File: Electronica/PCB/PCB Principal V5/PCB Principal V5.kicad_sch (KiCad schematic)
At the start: 17 parts, among them J1 Conexion Sensores, J12 TP, J2 Power Monster, J3 On/Off General, J4 Power Input 2, J5 IDC Placa Botones, J6 Power Input 1, SW1 On/Off Motores

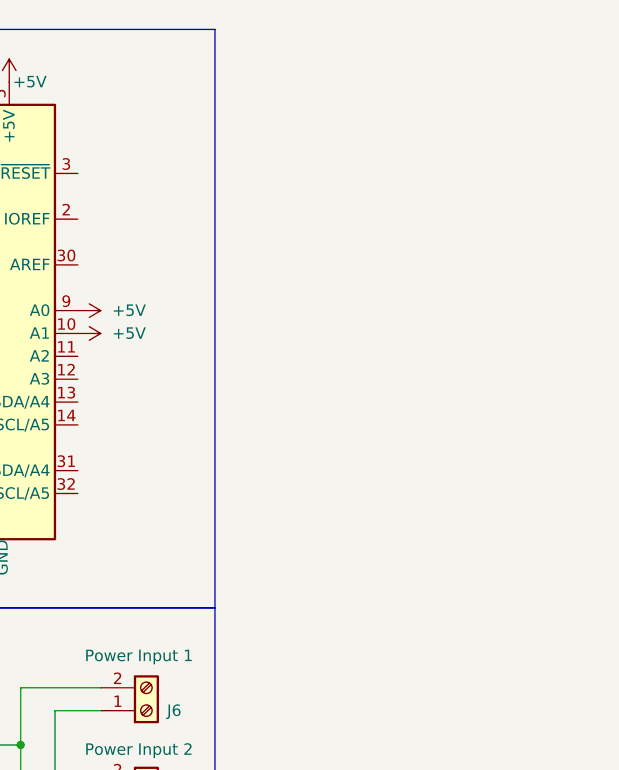
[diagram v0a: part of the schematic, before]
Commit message: ok
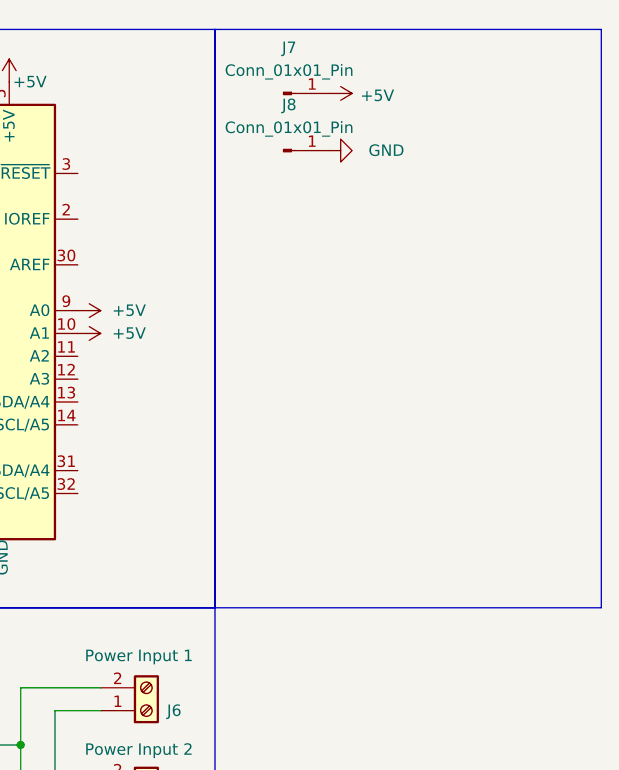
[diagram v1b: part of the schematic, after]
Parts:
- added J7, J8: Conn_01x01_Pin, Connector_PinHeader_2.54mm:PinHeader_1x01_P2.54mm_Vertical, symbol Connector:Conn_01x01_Pin
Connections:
- net +5V: now also J7.1 (Pin_1)
- net GND: now also J8.1 (Pin_1)

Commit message: .
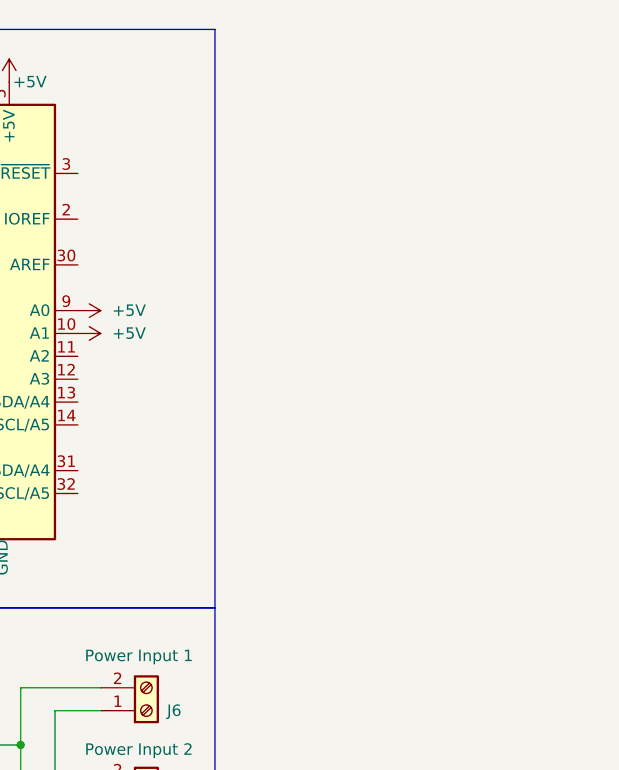
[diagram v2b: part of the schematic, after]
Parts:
- removed J7, J8: Conn_01x01_Pin, Connector_PinHeader_2.54mm:PinHeader_1x01_P2.54mm_Vertical, symbol Connector:Conn_01x01_Pin

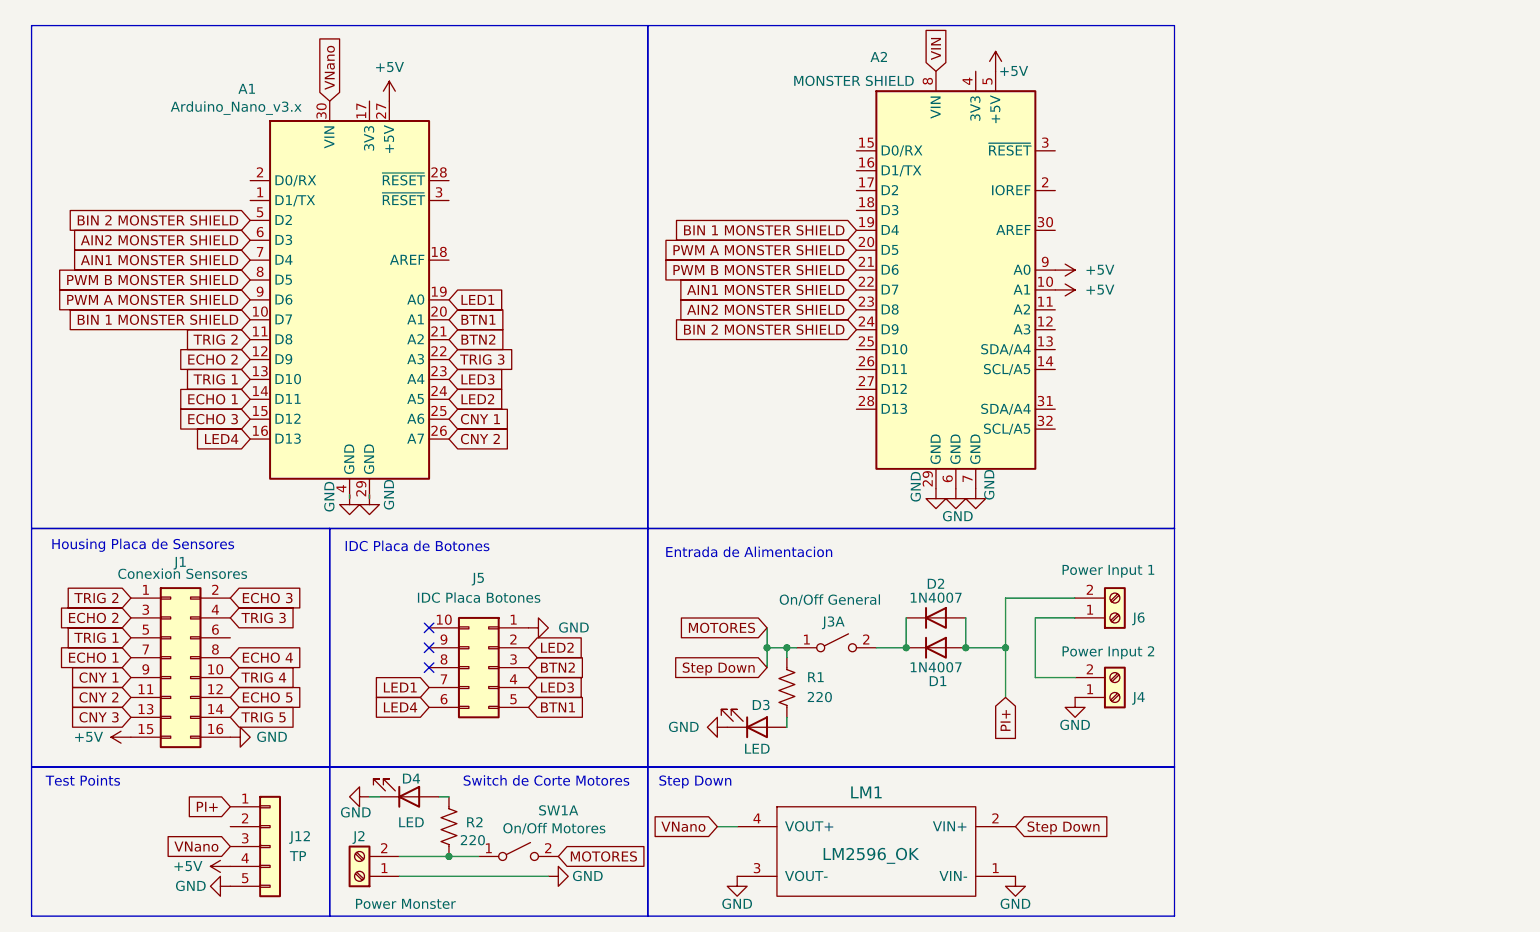
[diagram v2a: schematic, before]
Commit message: PCB V5 LINDA HERMOSA DIVINA
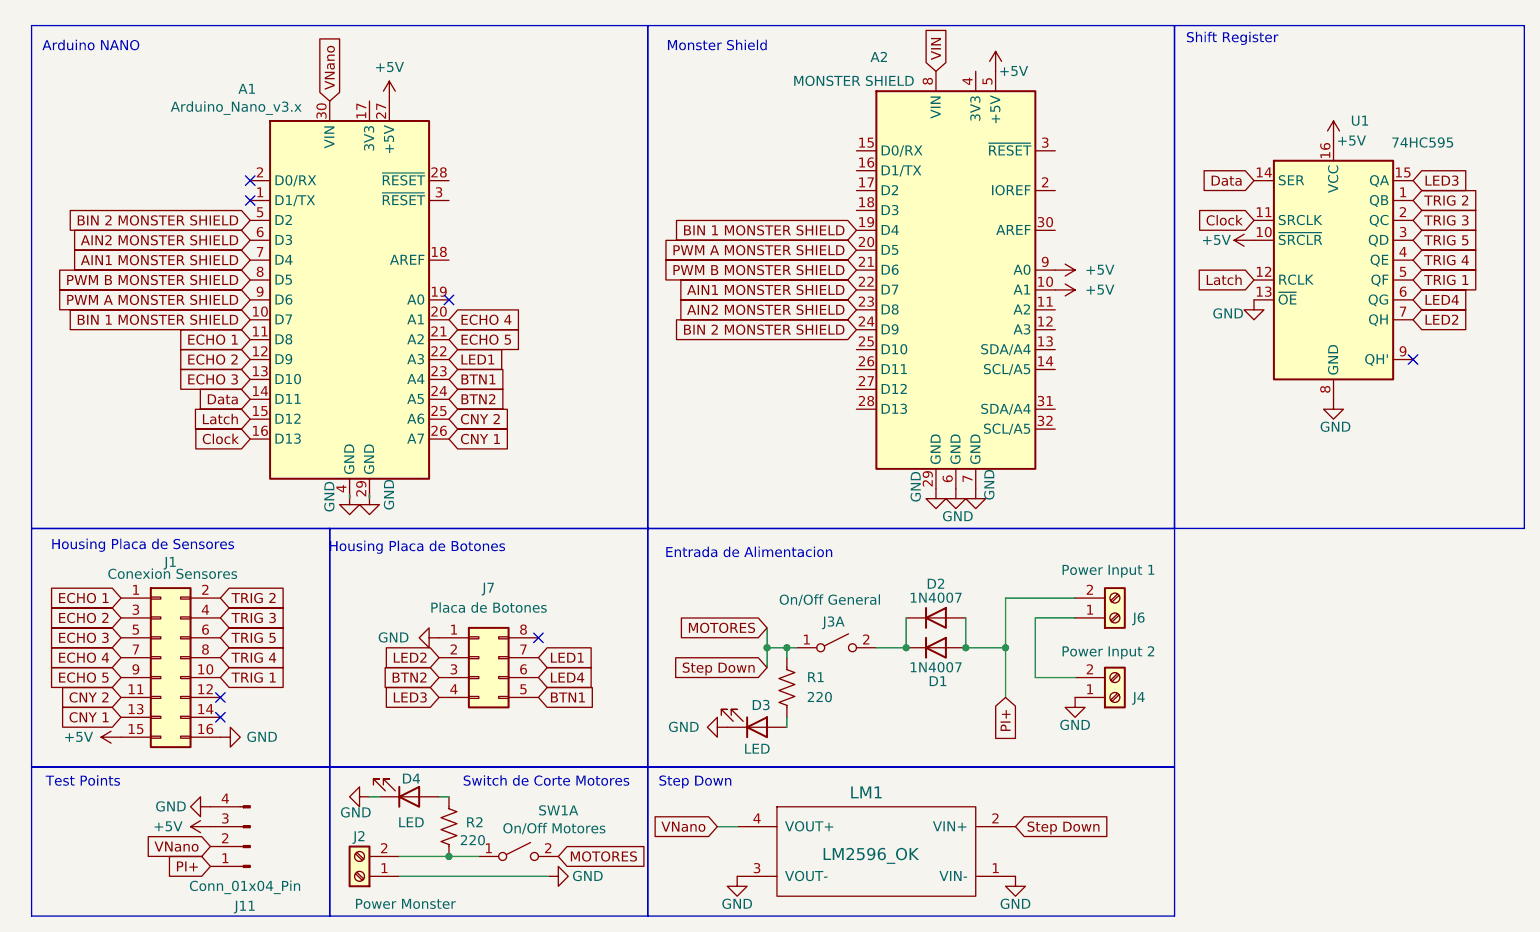
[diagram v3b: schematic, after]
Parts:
- removed J12: TP, Connector_PinHeader_2.54mm:PinHeader_1x05_P2.54mm_Vertical, symbol Connector_Generic:Conn_01x05
- removed J5: IDC Placa Botones, Connector_PinHeader_2.54mm:PinHeader_2x05_P2.54mm_Horizontal, symbol Connector_Generic:Conn_02x05_Counter_Clockwise
- added J11: Conn_01x04_Pin, Connector_PinHeader_2.54mm:PinHeader_1x04_P2.54mm_Vertical, symbol Connector:Conn_01x04_Pin
- added J7: Placa de Botones, Connector_PinHeader_2.54mm:PinHeader_2x04_P2.54mm_Horizontal, symbol Connector_Generic:Conn_02x04_Counter_Clockwise
- added U1: 74HC595, 74HC595N_DIP16_:DIP16-2.54-20.32X5.84MM, symbol 74xx:74HC595
- LM1: footprint Step Down:LM2596_correctedMeas -> StepDown:StepDown
- SW1: footprint Button_Switch_THT:SW_Slide_SPDT_Angled_CK_OS102011MA1Q -> Button_Switch_THT:SW_Slide_SPDT_Straight_CK_OS102011MS2Q
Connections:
- net CNY 3 is gone; now on net CNY 1: J1.13 (Pin_13)
- net +5V: now also J11.3 (Pin_3), U1.10 (~{SRCLR}), U1.16 (VCC)
- net BTN1: now also A1.23 (A4), J7.5 (Pin_5); no longer A1.20 (A1)
- net BTN2: now also A1.24 (A5), J7.3 (Pin_3); no longer A1.21 (A2)
- net CNY 1: now also A1.26 (A7); no longer A1.25 (A6), J1.9 (Pin_9)
- net CNY 2: now also A1.25 (A6); no longer A1.26 (A7)
- net ECHO 1: now also A1.11 (D8), J1.1 (Pin_1); no longer A1.14 (D11), J1.7 (Pin_7)
- net ECHO 3: now also A1.13 (D10), J1.5 (Pin_5); no longer A1.15 (D12), J1.2 (Pin_2)
- net ECHO 4: now also A1.20 (A1), J1.7 (Pin_7); no longer J1.8 (Pin_8)
- net ECHO 5: now also A1.21 (A2), J1.9 (Pin_9); no longer J1.12 (Pin_12)
- net GND: now also J11.4 (Pin_4), J7.1 (Pin_1), U1.13 (~{OE}), U1.8 (GND)
- net LED1: now also A1.22 (A3), J7.7 (Pin_7); no longer A1.19 (A0)
- net LED2: now also J7.2 (Pin_2), U1.7 (QH); no longer A1.24 (A5)
- net LED3: now also J7.4 (Pin_4), U1.15 (QA); no longer A1.23 (A4)
- net LED4: now also J7.6 (Pin_6), U1.6 (QG); no longer A1.16 (D13)
- net PI+: now also J11.1 (Pin_1)
- net TRIG 1: now also J1.10 (Pin_10), U1.5 (QF); no longer A1.13 (D10), J1.5 (Pin_5)
- net TRIG 2: now also J1.2 (Pin_2), U1.1 (QB); no longer A1.11 (D8), J1.1 (Pin_1)
- net TRIG 3: now also U1.2 (QC); no longer A1.22 (A3)
- net TRIG 4: now also J1.8 (Pin_8), U1.4 (QE); no longer J1.10 (Pin_10)
- net TRIG 5: now also J1.6 (Pin_6), U1.3 (QD); no longer J1.14 (Pin_14)
- net VNano: now also J11.2 (Pin_2)
- new net Clock: A1.16 (D13), U1.11 (SRCLK)
- new net Data: A1.14 (D11), U1.14 (SER)
- new net Latch: A1.15 (D12), U1.12 (RCLK)
- no-connect marks 3 -> 7
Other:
- note added: "Arduino NANO"
- note added: "Housing Placa de Botones"
- note added: "Monster Shield"
- note added: "Shift Register"
- note removed: "IDC Placa de Botones"

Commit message: PCB Principal V5 terminada
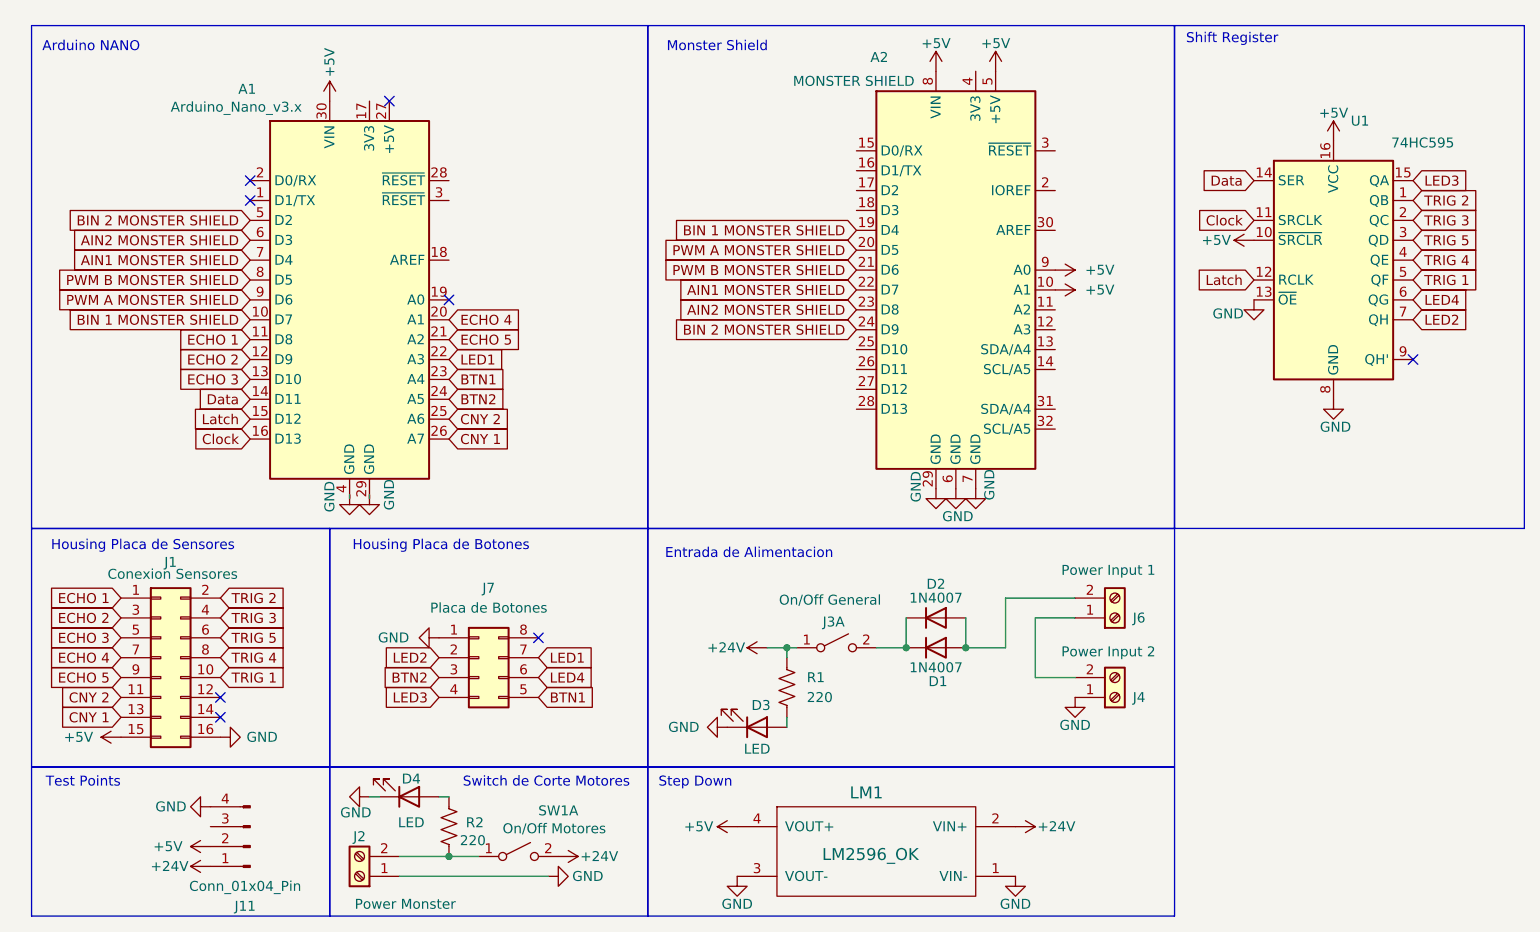
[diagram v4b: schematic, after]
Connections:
- net VIN is gone; now on net +5V: A2.8 (VIN)
- net VNano is gone; now on net +5V: A1.30 (VIN), J11.2 (Pin_2), LM1.4 (VOUT+)
- net +5V: no longer A1.27 (+5V), J11.3 (Pin_3)
- net MOTORES renamed +24V
- net +24V: now also J11.1 (Pin_1)
- net PI+: no longer names the net of D1.2 (A), D2.2 (A), J6.2 (Pin_2)
- net PI+: no longer J11.1 (Pin_1)
- no-connect marks 7 -> 8
